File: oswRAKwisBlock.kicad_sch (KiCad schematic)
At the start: 33 parts, among them J1 WisBlock, J2 0524352471, J4 10114830-10102LF, J5 USB micro, Q1 SI1308EDL-T1-GE3, U1 MCP73811T-420I/OT

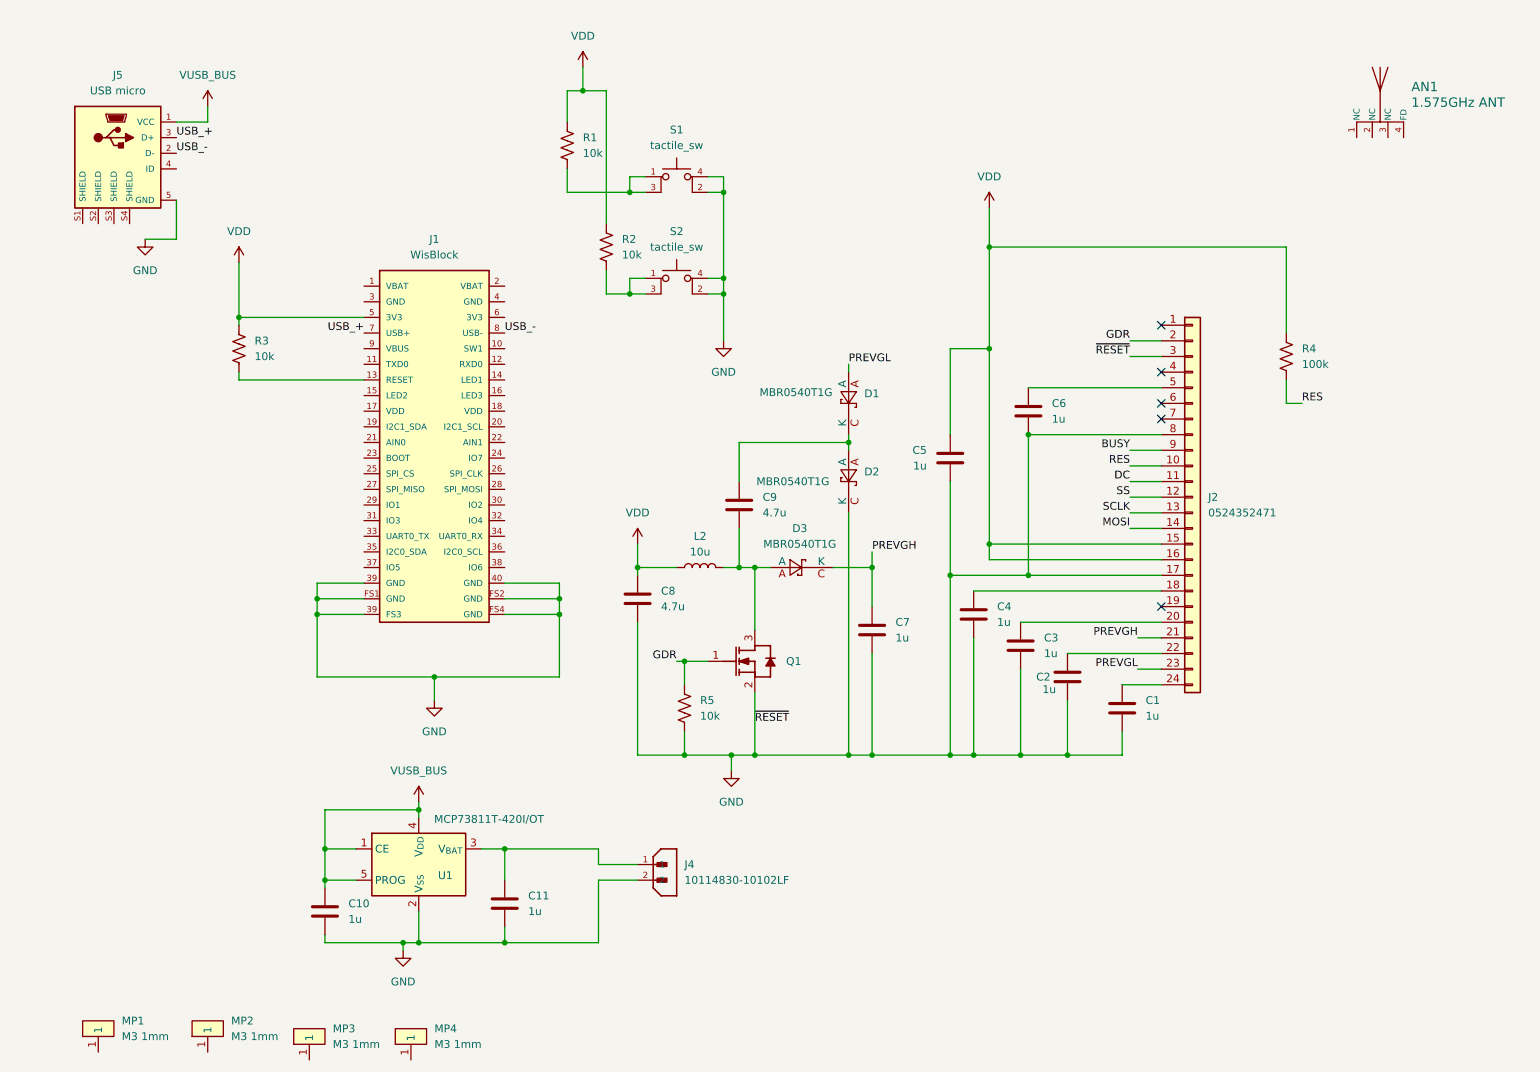
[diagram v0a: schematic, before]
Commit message: Working on things.
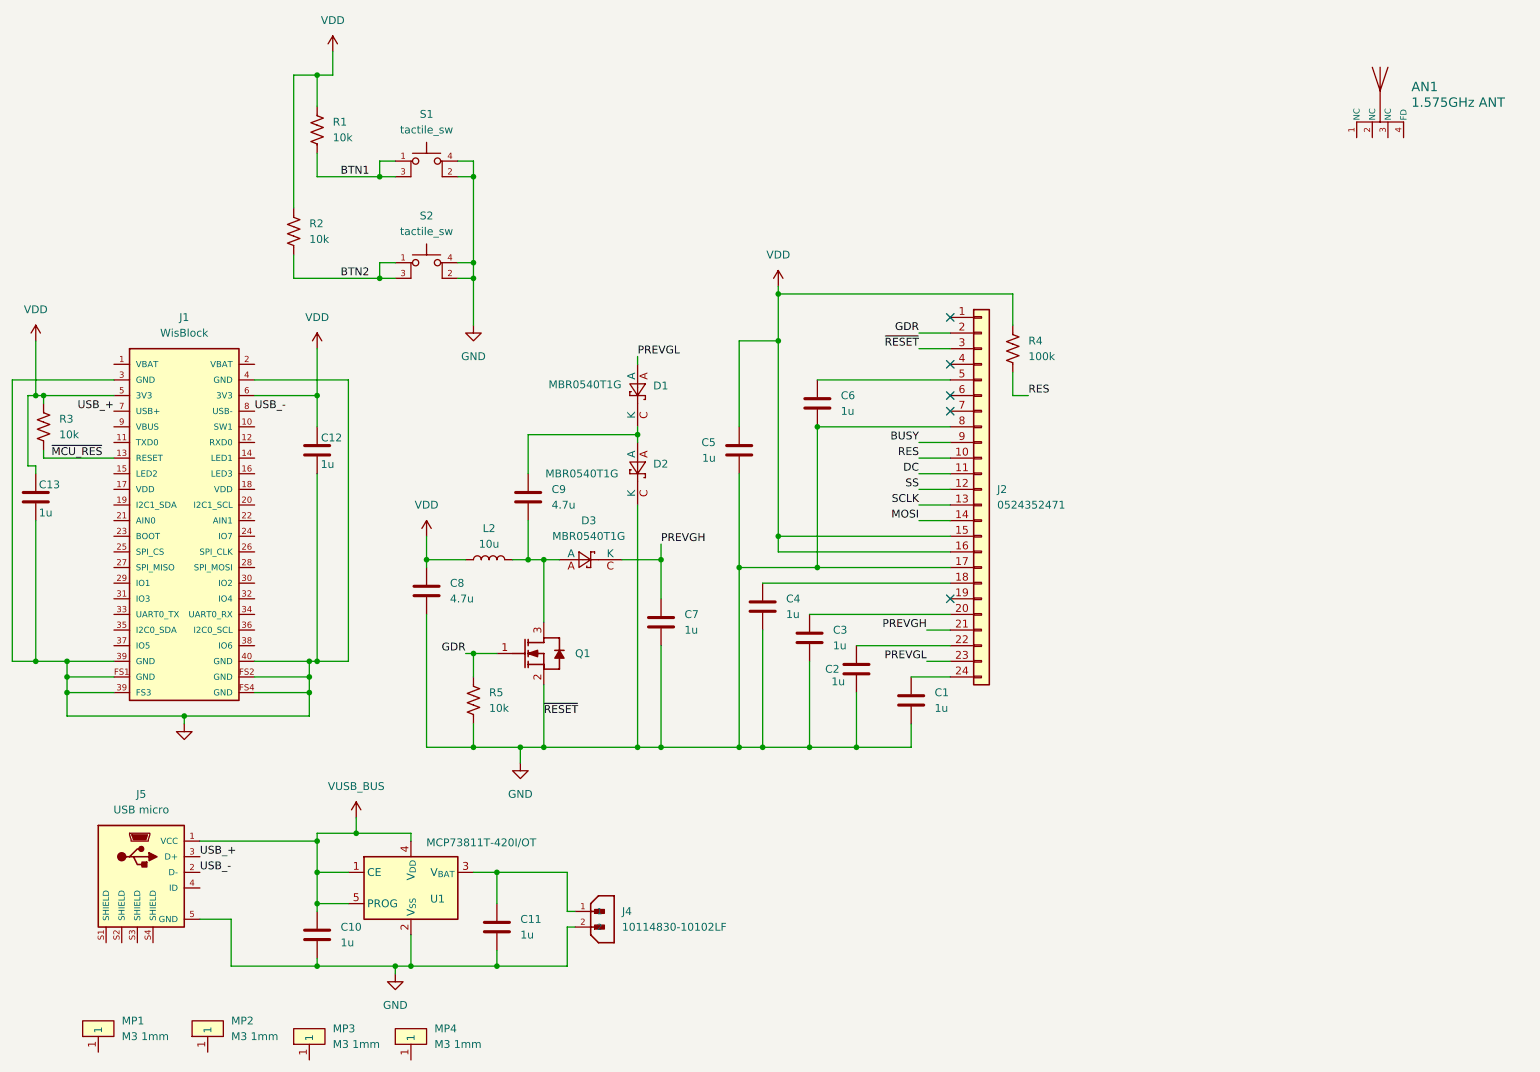
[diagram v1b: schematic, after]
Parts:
- added C12, C13: 1u, AllardChip:CAPC100X50X60L25L, symbol AllardPassive:C10A72-10000
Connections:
- net GND: now also J1.3 (GND), J1.4 (GND), C12.2, C13.2
- net VDD: now also J1.6 (3V3), C12.1, C13.1
- net BTN1: now reaches R1.2, S1.1, S1.3 (K)
- net ~{MCU_RES}: now reaches J1.13 (RESET), R3.2
- net BTN2: now reaches R2.2, S2.1, S2.3 (K)
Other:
- moved on the sheet: C1, C10, C11, C2, C3, C4, C5, C6, C7, C8, C9, D1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
